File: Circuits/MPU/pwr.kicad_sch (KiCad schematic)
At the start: 0 parts

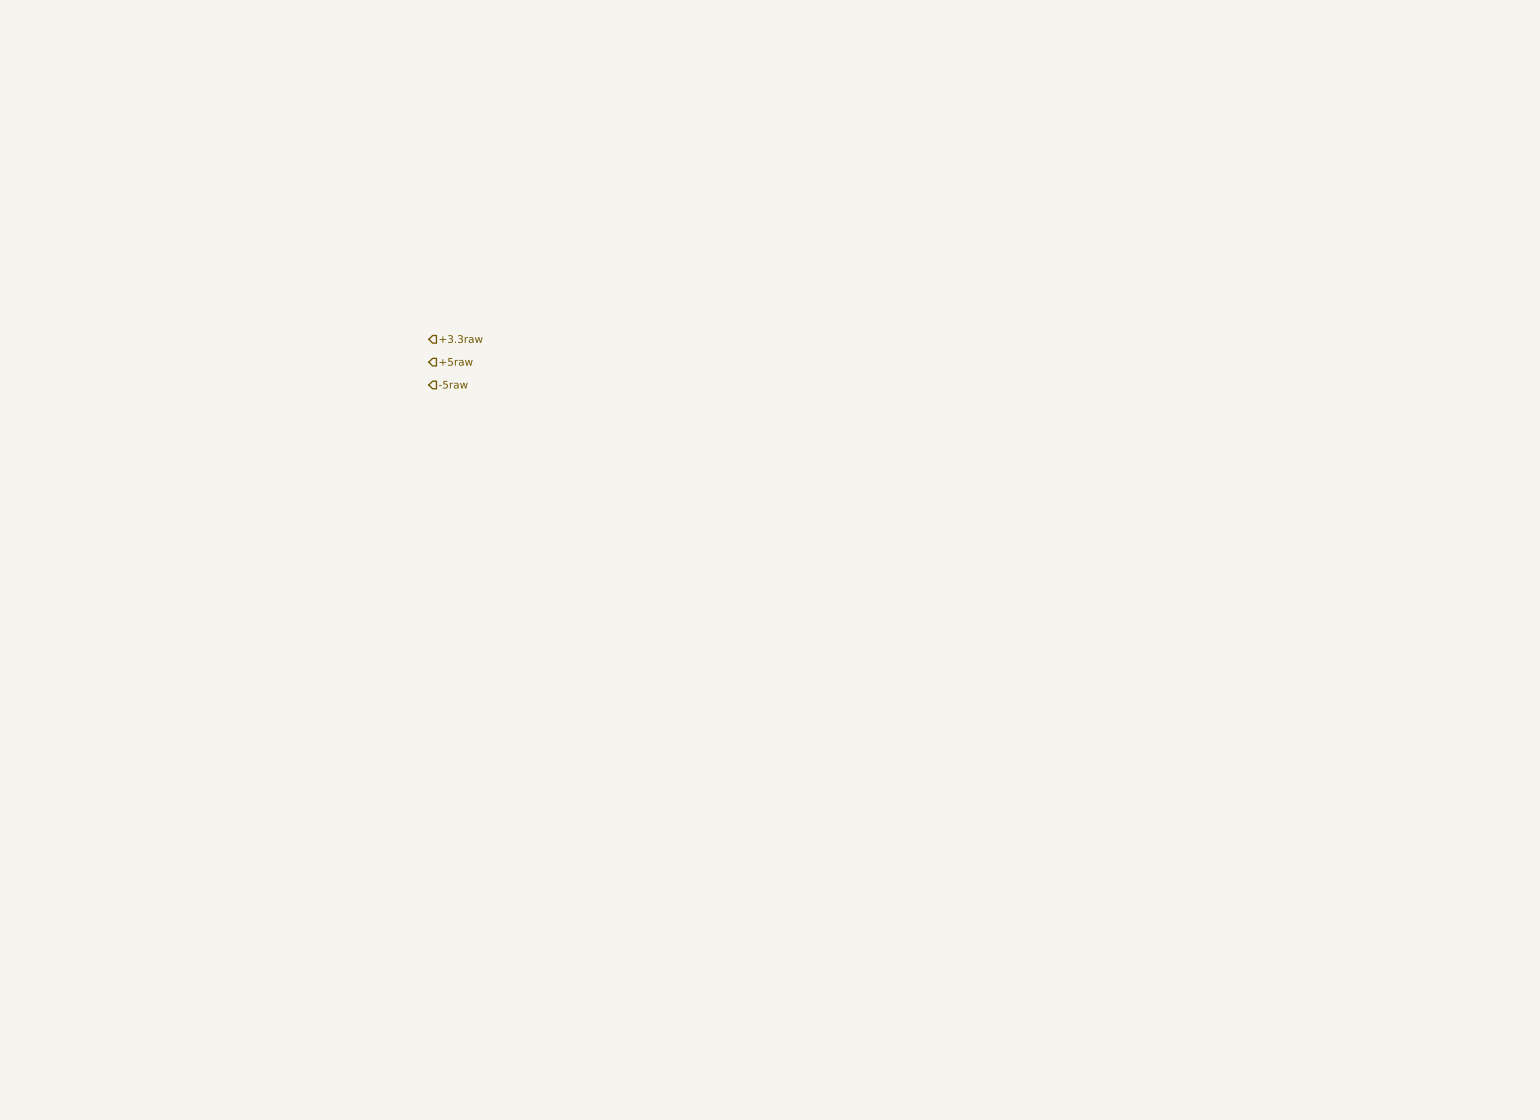
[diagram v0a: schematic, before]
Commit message: more transcription
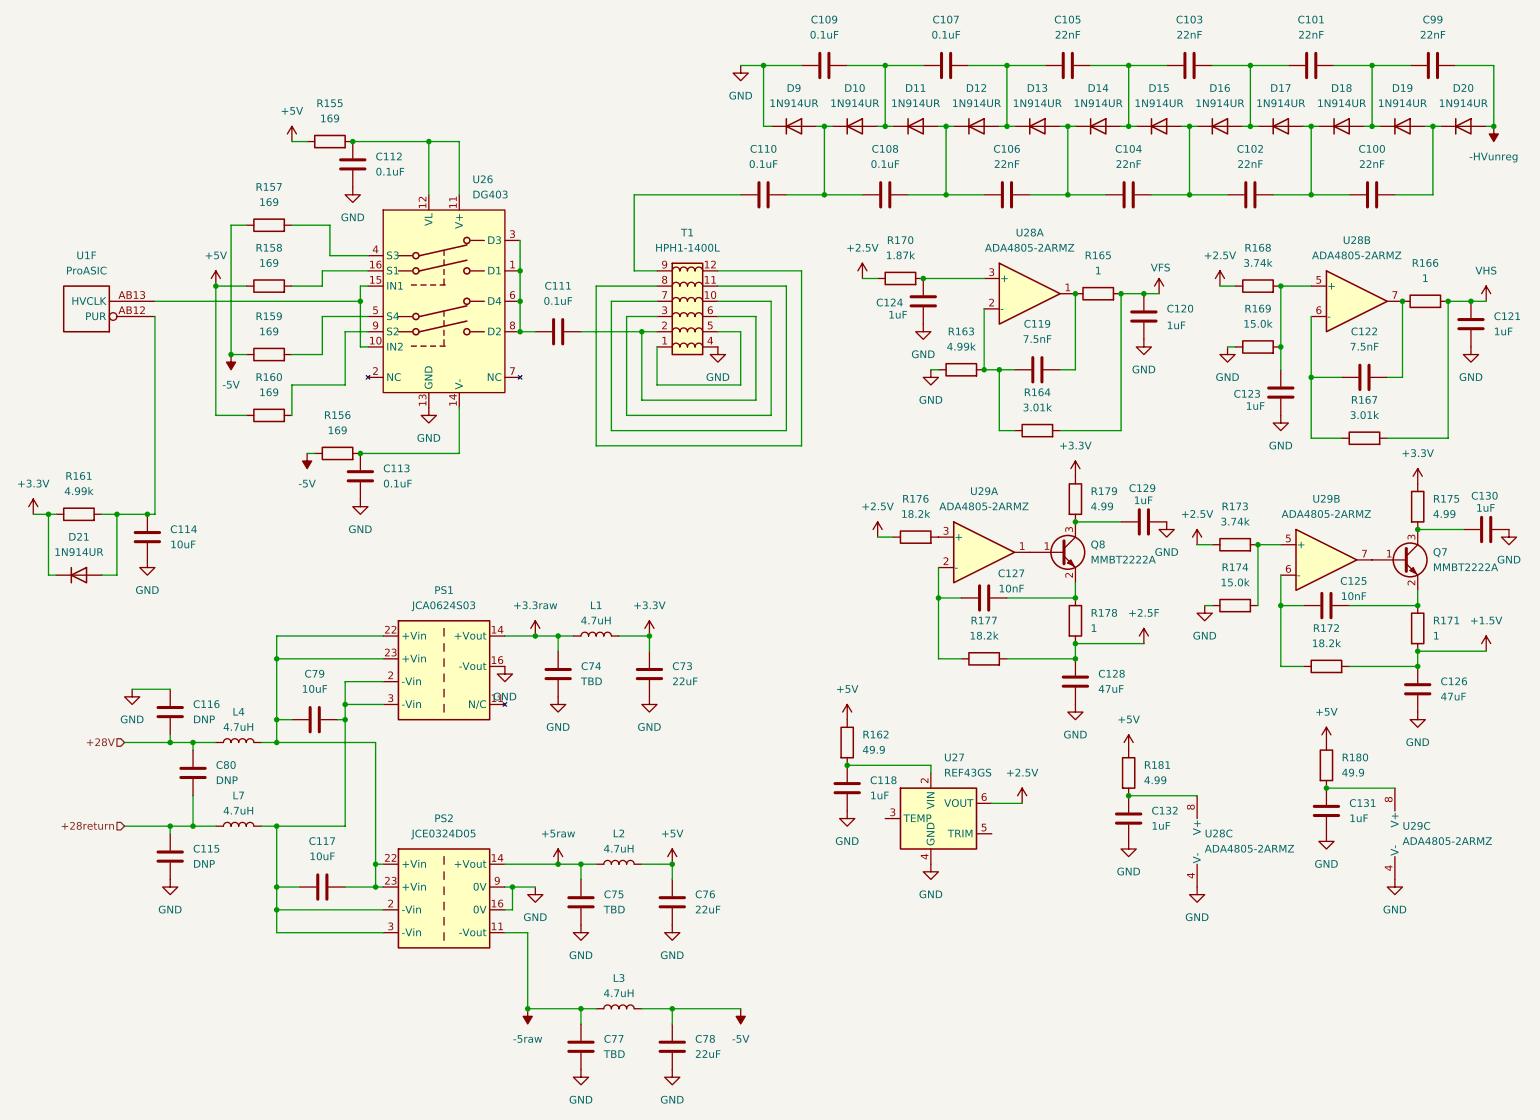
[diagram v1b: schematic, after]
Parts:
- added 	U1: ProASIC, Package_BGA:BGA-484_23.0x23.0mm_Layout22x22_P1.0mm, symbol QuERI_FPGA:ProASIC
- added C100, C101, C102, C103, C104, C105, C106, C99: 22nF, Capacitor_SMD:C_0603_1608Metric, symbol QuERI_symbols:Csmall
- added C107, C108, C109, C110, C111: 0.1uF, Capacitor_SMD:C_0805_2012Metric, symbol QuERI_symbols:C
- added C112, C113: 0.1uF, Capacitor_SMD:C_0603_1608Metric, symbol QuERI_symbols:Csmall
- added C114: 10uF, Capacitor_SMD:C_0805_2012Metric, symbol QuERI_symbols:C
- added C115, C116, C80: DNP, Capacitor_SMD:C_1210_3225Metric, symbol QuERI_symbols:C
- added C117, C79: 10uF, Capacitor_SMD:C_1210_3225Metric, symbol QuERI_symbols:C
- added C118, C120, C121, C123, C124, C129, C130, C131, C132: 1uF, Capacitor_SMD:C_0805_2012Metric, symbol QuERI_symbols:C
- added C119, C122: 7.5nF, Capacitor_SMD:C_0603_1608Metric, symbol QuERI_symbols:Csmall
- added C125, C127: 10nF, Capacitor_SMD:C_0603_1608Metric, symbol QuERI_symbols:Csmall
- added C126, C128: 47uF, Capacitor_SMD:C_1210_3225Metric, symbol QuERI_symbols:C
- added C73, C76, C78: 22uF, Capacitor_SMD:C_1210_3225Metric, symbol QuERI_symbols:C
- added C74, C75, C77: TBD, Capacitor_SMD:C_1210_3225Metric, symbol QuERI_symbols:C
- added D10, D11, D12, D13, D14, D15, D16, D17, D18, D19, D20, D21, D9: 1N914UR, Diode_SMD:D_MiniMELF, symbol QuERI_symbols:1N914UR
- added L1, L2, L3, L4, L7: 4.7uH, Inductor_SMD:L_1008_2520Metric, symbol Device:L
- added PS1: JCA0624S03, symbol QuERI_symbols:JCA0624S03
- added PS2: JCE0324D05, symbol QuERI_symbols:JCE0324D05
- added Q7, Q8: MMBT2222A, Package_TO_SOT_SMD:SOT-23, symbol Transistor_BJT:MMBT2222A
- added R155, R156, R157, R158, R159, R160: 169, Resistor_SMD:R_1206_3216Metric, symbol Device:R
- added R161, R163: 4.99k, Resistor_SMD:R_0603_1608Metric, symbol QuERI_symbols:Rlowp
- added R162, R180: 49.9, Resistor_SMD:R_0603_1608Metric, symbol QuERI_symbols:Rlowp
- added R164, R167: 3.01k, Resistor_SMD:R_0603_1608Metric, symbol QuERI_symbols:Rlowp
- added R165, R166, R171, R178: 1, Resistor_SMD:R_0603_1608Metric, symbol QuERI_symbols:Rlowp
- added R168, R173: 3.74k, Resistor_SMD:R_0603_1608Metric, symbol QuERI_symbols:Rlowp
- added R169, R174: 15.0k, Resistor_SMD:R_0603_1608Metric, symbol QuERI_symbols:Rlowp
- added R170: 1.87k, Resistor_SMD:R_0603_1608Metric, symbol QuERI_symbols:Rlowp
- added R172, R176, R177: 18.2k, Resistor_SMD:R_0603_1608Metric, symbol QuERI_symbols:Rlowp
- added R175, R179, R181: 4.99, Resistor_SMD:R_0603_1608Metric, symbol QuERI_symbols:Rlowp
- added T1: HPH1-1400L, symbol QuERI_symbols:Hexapath
- added U26: DG403, Package_SO:SOIC-16_3.9x9.9mm_P1.27mm, symbol QuERI_symbols:DG403
- added U27: REF43GS, Package_SO:SOIC-8_3.9x4.9mm_P1.27mm, symbol QuERI_symbols:REF43GS
- added U28, U29: ADA4805-2ARMZ, Package_SO:MSOP-8_3x3mm_P0.65mm, symbol QuERI_symbols:ADA4805-2ARMZ
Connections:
- net +3.3raw: now also C74.1, L1.1, PS1.14 (+Vout)
- net +5raw: now also C75.1, L2.1, PS2.14 (+Vout)
- net -5raw: now also C77.1, L3.1, PS2.11 (-Vout)
- new net: C107.1, C109.2, D10.2 (A), D11.1 (K)
- new net: C106.1, C108.2, D11.2 (A), D12.1 (K)
- new net: C112.1, R155.2, U26.11 (V+), U26.12 (VL)
- new net: C123.1, R168.2, R169.2, U28.5 (+)
- new net: R160.2, U26.9 (S2)
- new net: C131.1, R180.2, U29.8 (V+)
- new net: Q8.1 (B), U29.1
- new net: C127.2, R177.1, U29.2 (-)
- new net: R176.2, U29.3 (+)
- new net: C101.2, C99.1, D18.2 (A), D19.1 (K)
- new net: C105.1, C107.2, D12.2 (A), D13.1 (K)
- new net: C103.1, C105.2, D14.2 (A), D15.1 (K)
- new net: C119.2, R163.2, R164.1, U28.2 (-)
- new net: C104.1, C106.2, D13.2 (A), D14.1 (K)
- new net: C102.1, C104.2, D15.2 (A), D16.1 (K)
- new net: C118.1, R162.2, U27.2 (VIN)
- new net: C125.1, Q7.2 (E), R171.1
- new net: C125.2, R172.1, U29.6 (-)
- new net: R173.2, R174.2, U29.5 (+)
- new net: C117.1, C79.2, L7.2, PS1.2 (-Vin), PS1.3 (-Vin), PS2.2 (-Vin), PS2.3 (-Vin)
- new net: C117.2, C79.1, L4.2, PS1.22 (+Vin), PS1.23 (+Vin), PS2.22 (+Vin), PS2.23 (+Vin)
- new net: C101.1, C103.2, D16.2 (A), D17.1 (K)
- new net: C100.1, C102.2, D17.2 (A), D18.1 (K)
- new net: C108.1, C110.2, D10.1 (K), D9.2 (A)
- new net: C127.1, Q8.2 (E), R178.1
- new net: C132.1, R181.2, U28.8 (V+)
- new net: Q7.1 (B), U29.7
- new net: C129.1, Q8.3 (C), R179.2
- new net: R159.2, U26.5 (S4)
- new net: C110.1, T1.9
- new net: R158.2, U26.16 (S1)
- new net: C100.2, D19.2 (A), D20.1 (K)
- new net: C130.1, Q7.3 (C), R175.2
- new net: C119.1, R165.1, U28.1
- new net: C124.1, R170.2, U28.3 (+)
- new net: C111.1, U26.1 (D1), U26.3 (D3), U26.6 (D4), U26.8 (D2)
- new net: C111.2, T1.2, T1.6
- new net: 	U1.AB12 (PUR), C114.1, D21.2 (A), R161.2
- new net: 	U1.AB13 (HVCLK), U26.10 (IN2), U26.15 (IN1)
- new net: C122.2, R167.1, U28.6 (-)
- new net: C122.1, R166.1, U28.7
- new net: C113.1, R156.2, U26.14 (V-)
- new net: R157.2, U26.4 (S3)
- new net: T1.1, T1.5
- new net: T1.10, T1.3
- new net: T1.11, T1.7
- new net: T1.12, T1.8
- new net +1.5V: C126.1, R171.2, R172.2
- new net +2.5F: C128.1, R177.2, R178.2
- new net +2.5V: R168.1, R170.1, R173.1, R176.1, U27.6 (VOUT)
- new net +28V: C116.2, C80.1, L4.1
- new net +28return: C115.1, C80.2, L7.1
- new net +3.3V: C73.1, D21.1 (K), L1.2, R161.1, R175.1, R179.1
- new net +5V: C76.1, L2.2, R155.1, R158.1, R160.1, R162.1, R180.1, R181.1
- new net -5V: C78.1, L3.2, R156.1, R157.1, R159.1
- new net -HVunreg: C99.2, D20.2 (A)
- new net GND: C109.1, C112.2, C113.2, C114.2, C115.2, C116.1, C118.2, C120.2, C121.2, C123.2, C124.2, C126.2, C128.2, C129.2, C130.2, C131.2, C132.2, C73.2, C74.2, C75.2, C76.2, C77.2, C78.2, D9.1 (K), PS1.16 (-Vout), PS2.16 (0V), PS2.9 (0V), R163.1, R169.1, R174.1, T1.4, U26.13 (GND), U27.4 (GND), U28.4 (V-), U29.4 (V-)
- new net VFS: C120.1, R164.2, R165.2
- new net VHS: C121.1, R166.2, R167.2
